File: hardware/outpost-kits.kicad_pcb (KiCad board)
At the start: 2 copper layers, 102.7 x 102.3 mm, 19 parts, among them J1 PROBE, SW1 ROLL, U1 NE555N, U2 CD4026, U3 SM420561N, U4 LM3915N

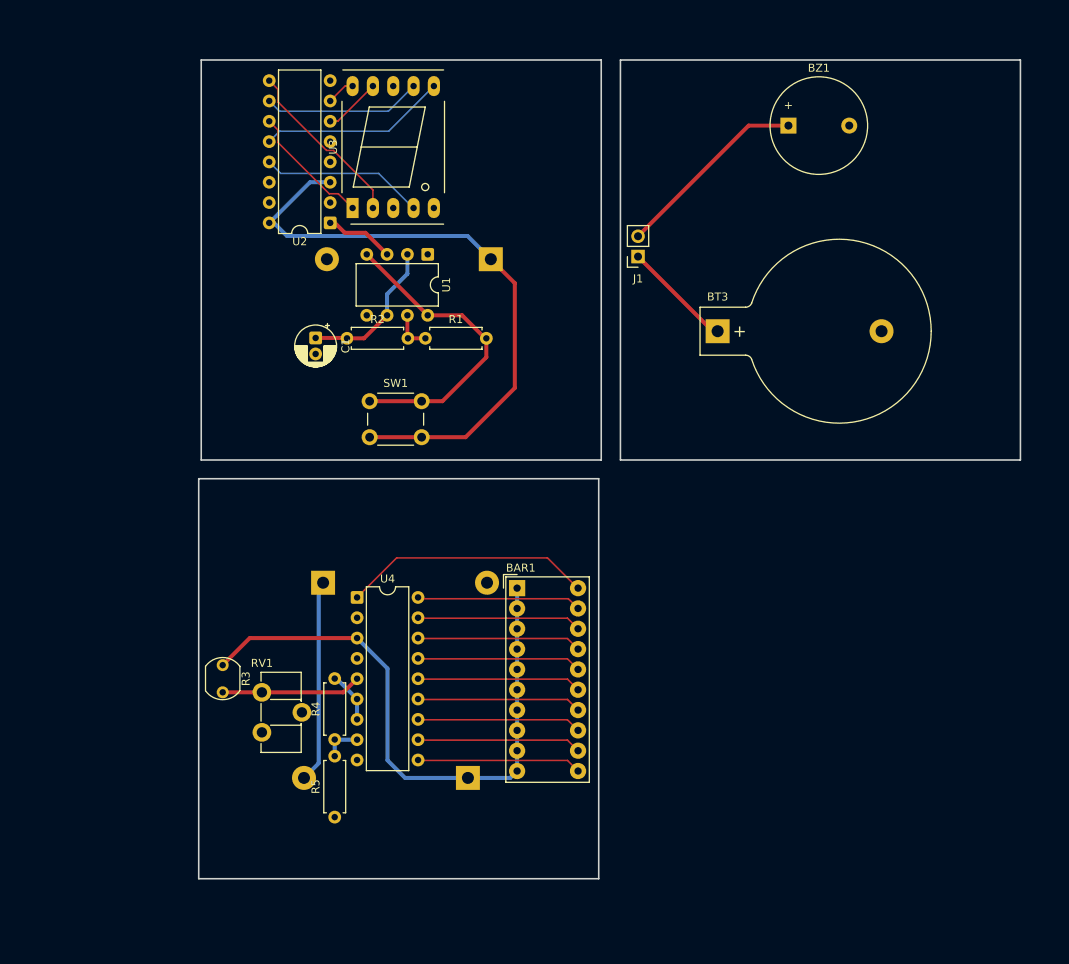
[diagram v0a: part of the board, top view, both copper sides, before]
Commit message: done v1?
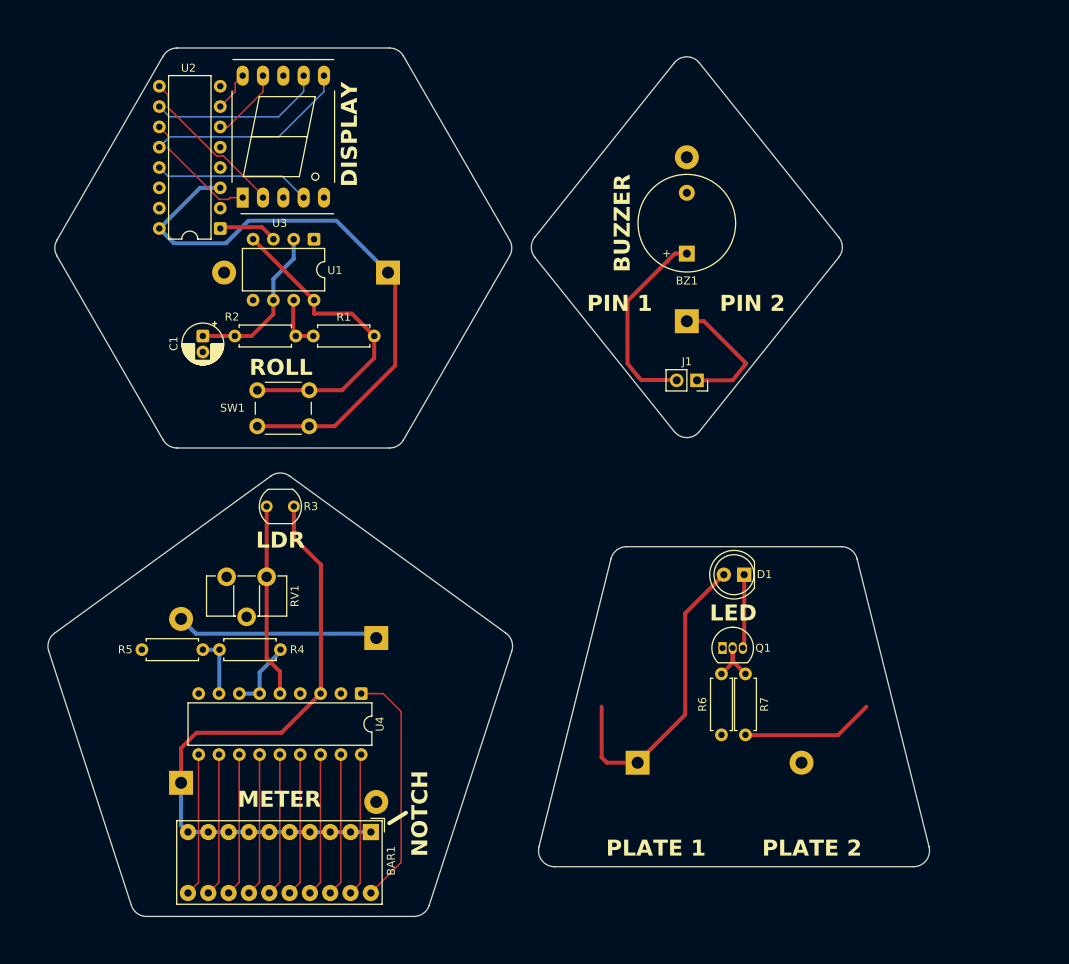
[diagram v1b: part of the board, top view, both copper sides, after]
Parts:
- added BT5: CR2032, Battery:BatteryHolder_Keystone_103_1x20mm, B.Cu at (155.1, 123.8)
- added D1: LED, LED_THT:LED_D5.0mm_FlatTop, F.Cu at (168.4, 100.3)
- added Q1: 2N3904, Package_TO_SOT_THT:TO-92_Inline, F.Cu at (165.7, 109.5)
- added R6: 100kR, Resistor_THT:R_Axial_DIN0207_L6.3mm_D2.5mm_P7.62mm_Horizontal, F.Cu at (165.5, 120.4)
- added R7: 10MR, Resistor_THT:R_Axial_DIN0207_L6.3mm_D2.5mm_P7.62mm_Horizontal, F.Cu at (168.5, 112.7)
- BT3: moved to B.Cu
- moved BT4 35.9 mm to (98.0, 126.4), turned to 90 degrees
- moved BAR1 35.5 mm to (121.7, 132.5), turned to -90 degrees
- moved R5 31.9 mm to (93.1, 109.7), turned to 0 degrees
- moved R3 21.7 mm to (112.1, 91.8), turned to 180 degrees
- moved BZ1 20.4 mm to (161.2, 60.2), turned to 90 degrees
- moved R4 18.3 mm to (102.8, 109.7), turned to 0 degrees
- moved J1 17.1 mm to (162.5, 76.0), turned to -90 degrees
- moved RV1 14.5 mm to (108.7, 100.6), turned to -90 degrees
- moved U1 14.3 mm to (114.6, 58.4)
- moved SW1 14.1 mm to (107.5, 77.3)
- moved C1 14.1 mm to (100.7, 70.5)
- moved R1 14.0 mm to (114.5, 70.5)
- moved R2 14.0 mm to (104.7, 70.5)
- moved U3 13.8 mm to (105.7, 53.2)
- moved U2 13.8 mm to (102.9, 57.1)
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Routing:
- net COND_3V: track 0.00 -> 39.1 mm
- net Net-(R7-Pad2): track 0.00 -> 16.6 mm
- net Net-(D1-K): track 0.00 -> 9.23 mm
- net Net-(Q1-B): track 0.00 -> 7.72 mm
- net Net-(U4-SIG): track 17.5 -> 24.1 mm
- net VU_6V: track 75.4 -> 78.8 mm
- net CONT_3V3: track 13.8 -> 16.8 mm
- net Net-(U4-REFADJ): track 4.88 -> 7.60 mm
- net Net-(U4-LED9): track 20.6 -> 17.9 mm
- net Net-(U4-LED7): track 20.6 -> 17.9 mm
- net Net-(U4-LED5): track 20.6 -> 17.9 mm
- net Net-(U4-LED3): track 20.6 -> 17.9 mm
- net Net-(U4-LED4): track 20.6 -> 17.9 mm
- net Net-(U4-LED2): track 20.6 -> 17.9 mm
- net Net-(U4-REFOUT): track 6.40 -> 9.11 mm
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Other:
- board size 102.7 x 102.3 mm -> 110.2 x 108.6 mm
- board text added: "BUZZER"
- board text added: "DISPLAY"
- board text added: "LDR"
- board text added: "LED"
- board text added: "METER"
- board text added: "NOTCH"
- board text added: "PIN 1"
- board text added: "PIN 2"
- board text added: "PLATE 1"
- board text added: "PLATE 2"
- board text added: "ROLL"

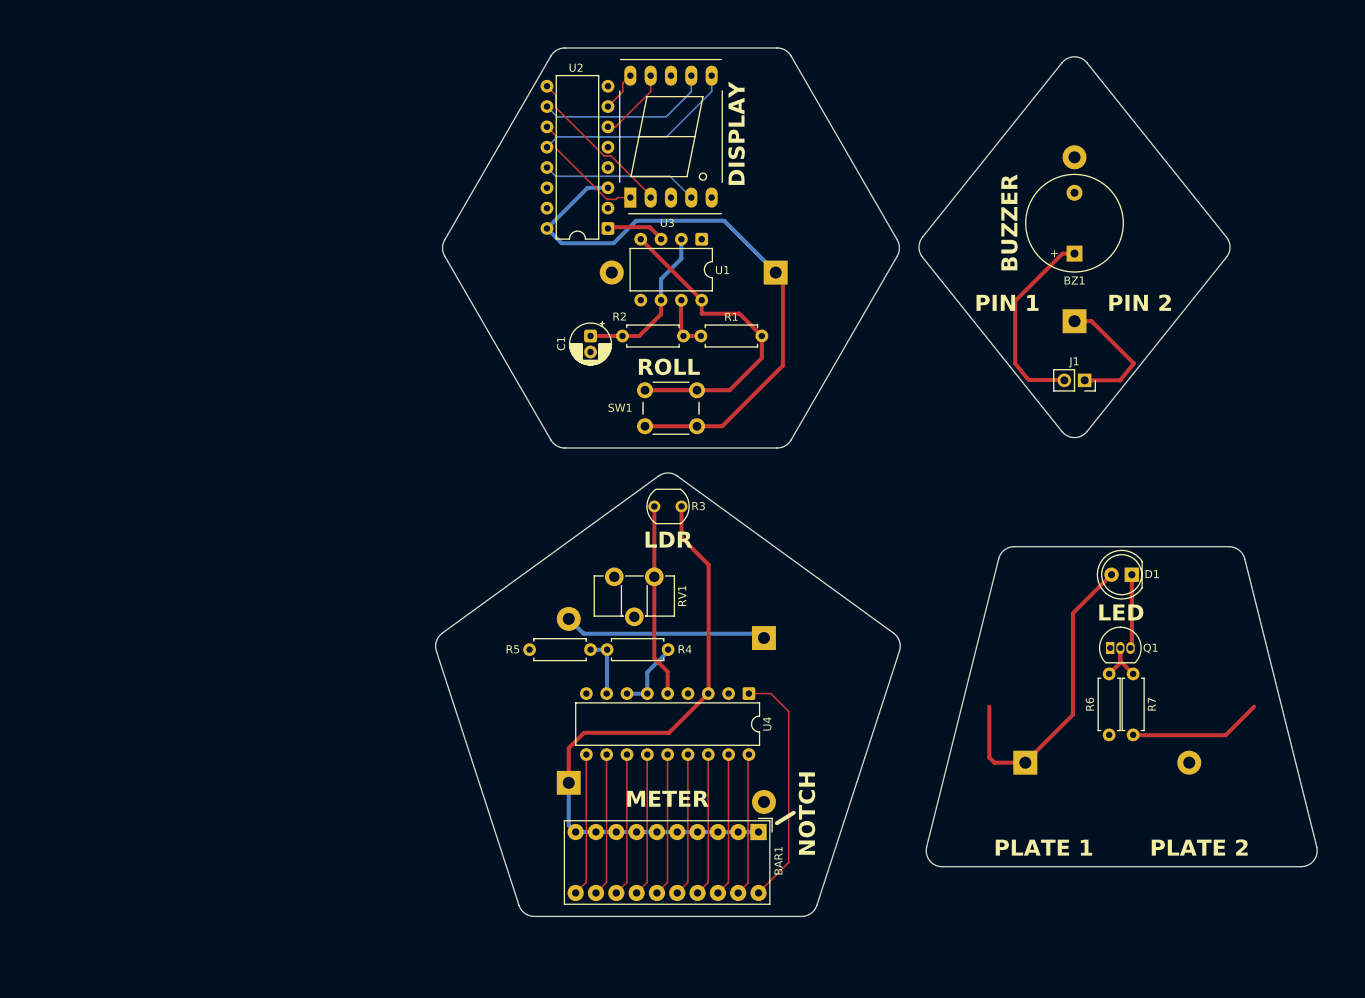
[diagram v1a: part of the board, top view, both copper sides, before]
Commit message: prod stuff
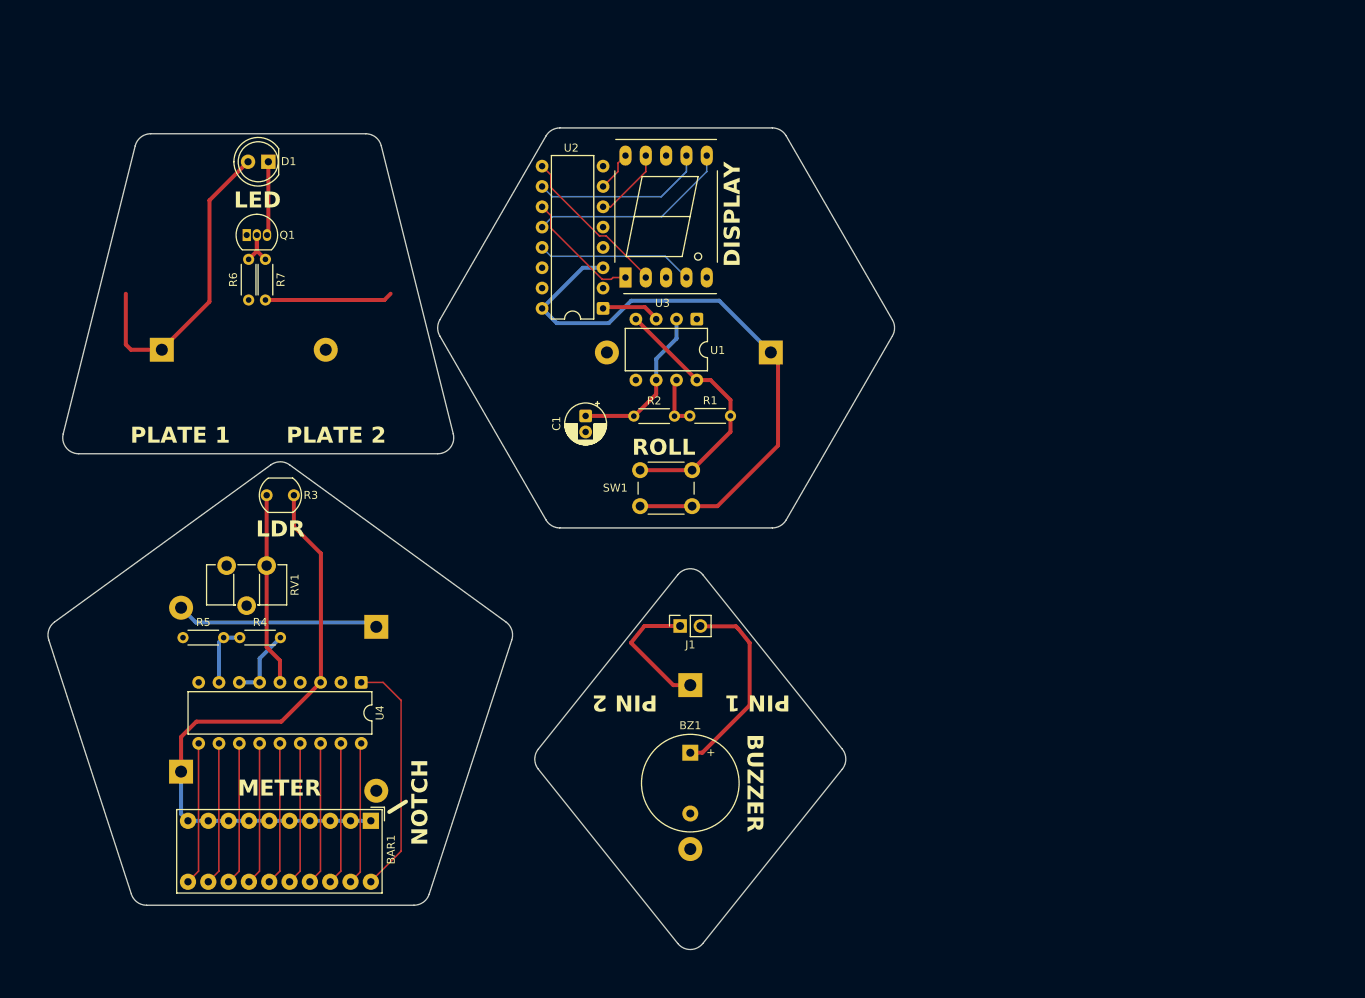
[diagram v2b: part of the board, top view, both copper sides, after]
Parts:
- added G***: LOGO, LOGO, B.Cu at (124.1, 118.7)
- added G***: LOGO, LOGO, B.Cu at (54.9, 134.6)
- added G***: LOGO, LOGO, B.Cu at (110.0, 51.8)
- added G***: LOGO, LOGO, B.Cu at (59.7, 52.9)
- R1, R2, R4, R5, R6, R7: footprint Resistor_THT:R_Axial_DIN0207_L6.3mm_D2.5mm_P7.62mm_Horizontal -> Resistor_THT:R_Axial_DIN0204_L3.6mm_D1.6mm_P5.08mm_Horizontal
- moved R6 120.5 mm to (58.0, 66.0)
- moved R7 120.2 mm to (60.1, 60.9)
- moved BT5 119.6 mm to (47.1, 72.2)
- moved D1 119.6 mm to (60.4, 48.7)
- moved Q1 119.6 mm to (57.7, 57.9)
- moved BZ1 78.7 mm to (113.2, 122.6), turned to -90 degrees
- moved BT3 66.2 mm to (113.2, 114.1), turned to -90 degrees
- moved J1 59.2 mm to (111.9, 106.8), turned to 90 degrees
- moved BT4 48.5 mm to (49.5, 125.0)
- moved R3 48.5 mm to (63.6, 90.4)
- moved BAR1 48.5 mm to (73.2, 131.1)
- moved BT1 48.5 mm to (73.9, 106.9)
- moved RV1 48.5 mm to (60.2, 99.2)
- moved U4 48.5 mm to (72.0, 113.8)
- moved R4 45.9 mm to (56.9, 108.2)
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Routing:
- net Net-(U1-VCC): track 40.2 -> 33.3 mm
- net Net-(Q1-B): track 7.72 -> 6.94 mm
- net Net-(R7-Pad2): track 16.6 -> 16.0 mm
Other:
- board size 110.2 x 108.6 mm -> 105.8 x 102.7 mm
